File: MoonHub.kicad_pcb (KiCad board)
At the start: 4 copper layers, 102 x 16.5 mm, 42 parts, among them J1 X1224WRS-04-LPV01, U1 AP22818AKBWT-7, U2 H5VU25U, U3 H5VU25U, U4 CH334U, U5 H5VU25U, Y1 12MHz

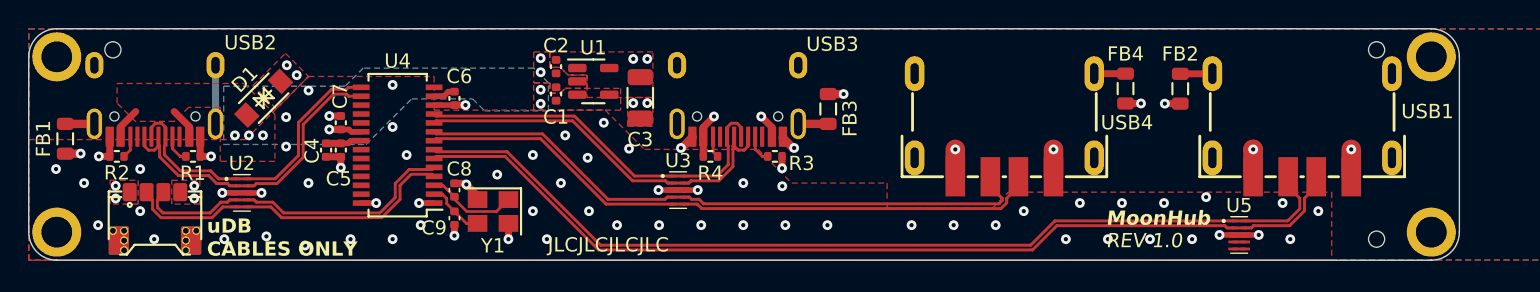
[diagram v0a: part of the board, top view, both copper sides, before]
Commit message: remove ferrites
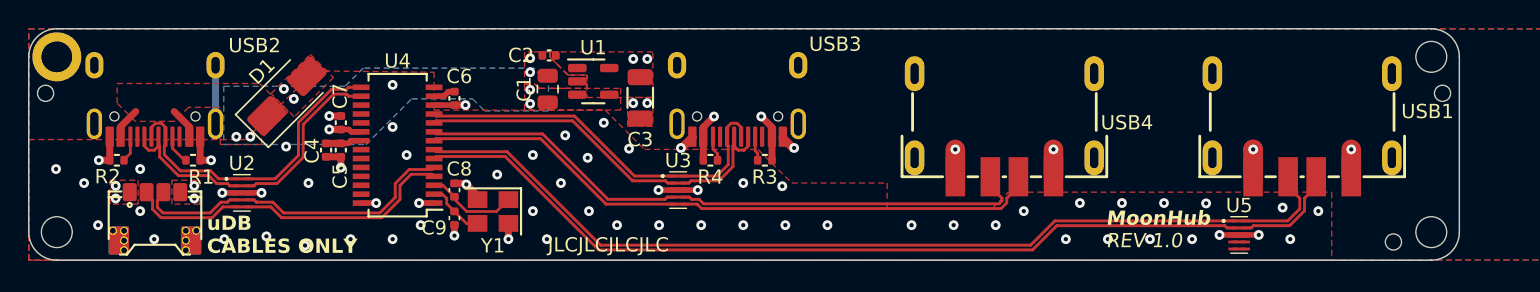
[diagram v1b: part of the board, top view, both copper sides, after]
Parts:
- removed FB1, FB2, FB3, FB4: 100R@100MHz, Inductor_SMD:L_0805_2012Metric
- C1: value 1u -> 10u; footprint Capacitor_SMD:C_0402_1005Metric -> Capacitor_SMD:C_0805_2012Metric
- D1: value SMF6.0CA -> SMAJ5.0A; footprint MoonHub:SOD-123FL_L2.8-W1.8-LS3.7-BI -> Diode_SMD:D_SMA
- H1, H3, H4: value MountingHole_Pad -> MountingHole; footprint MoonHub:Generic-Mounthole -> MountingHole:MountingHole_2.2mm_M2_ISO7380
- moved H3 98.0 mm to (100.0, 14.5)
- moved H4 98.0 mm to (2.00, 14.5)
- moved H5 5.71 mm to (1.20, 4.60)
- moved H6 5.63 mm to (100.8, 4.60)
- moved D1 1.66 mm to (18.4, 4.80), turned to 45 degrees
- moved H7 1.22 mm to (97.3, 15.2)
- moved C2 0.94 mm to (37.1, 1.90), turned to 180 degrees
- moved R3 0.77 mm to (52.5, 9.38)
- moved C1 0.69 mm to (37.0, 4.30)
- moved R1 0.28 mm to (11.7, 9.38)
- moved R2 0.28 mm to (6.28, 9.38)
- moved R4 0.28 mm to (48.6, 9.38)
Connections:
- D1 pad 1: GND -> +5V
- D1 pad 2: +5V -> GND
- J1 pad MP: GND -> GNDPWR
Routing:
- net GNDPWR: track 12.9 -> 4.18 mm
- net GND: track 33.9 -> 30.0 mm, vias 84 -> 78
- net VBUS: track 9.67 -> 10.8 mm, vias 9 -> 8
- net +5V: vias 6 -> 5
